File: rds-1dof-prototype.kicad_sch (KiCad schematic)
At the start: 10 parts, among them U1 Teensy4.0

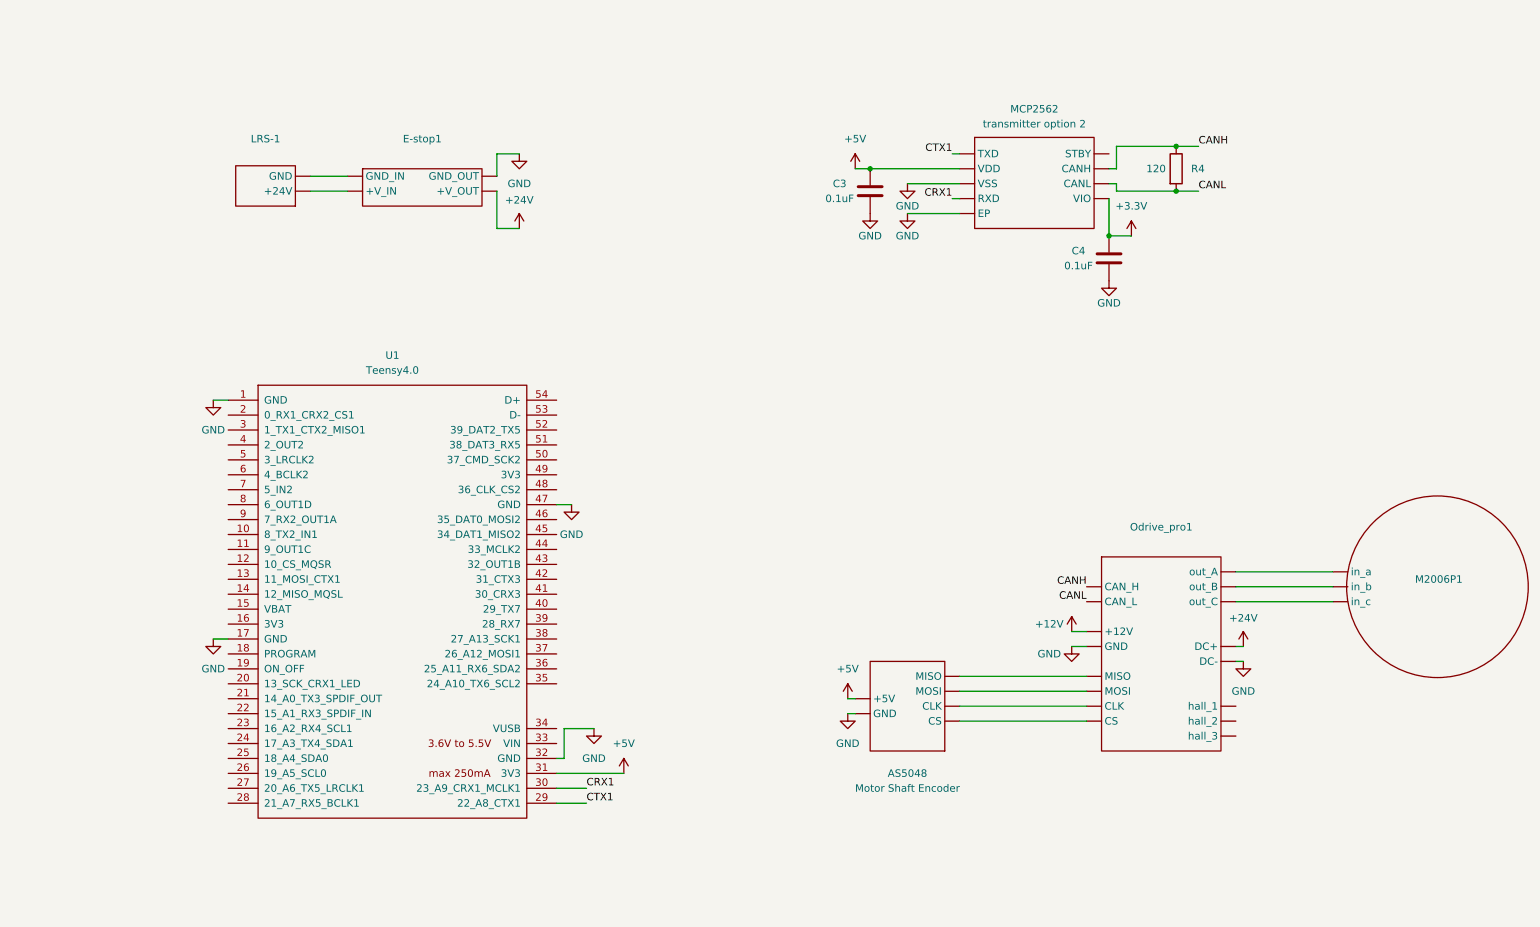
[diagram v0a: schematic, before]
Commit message: Formatting updates
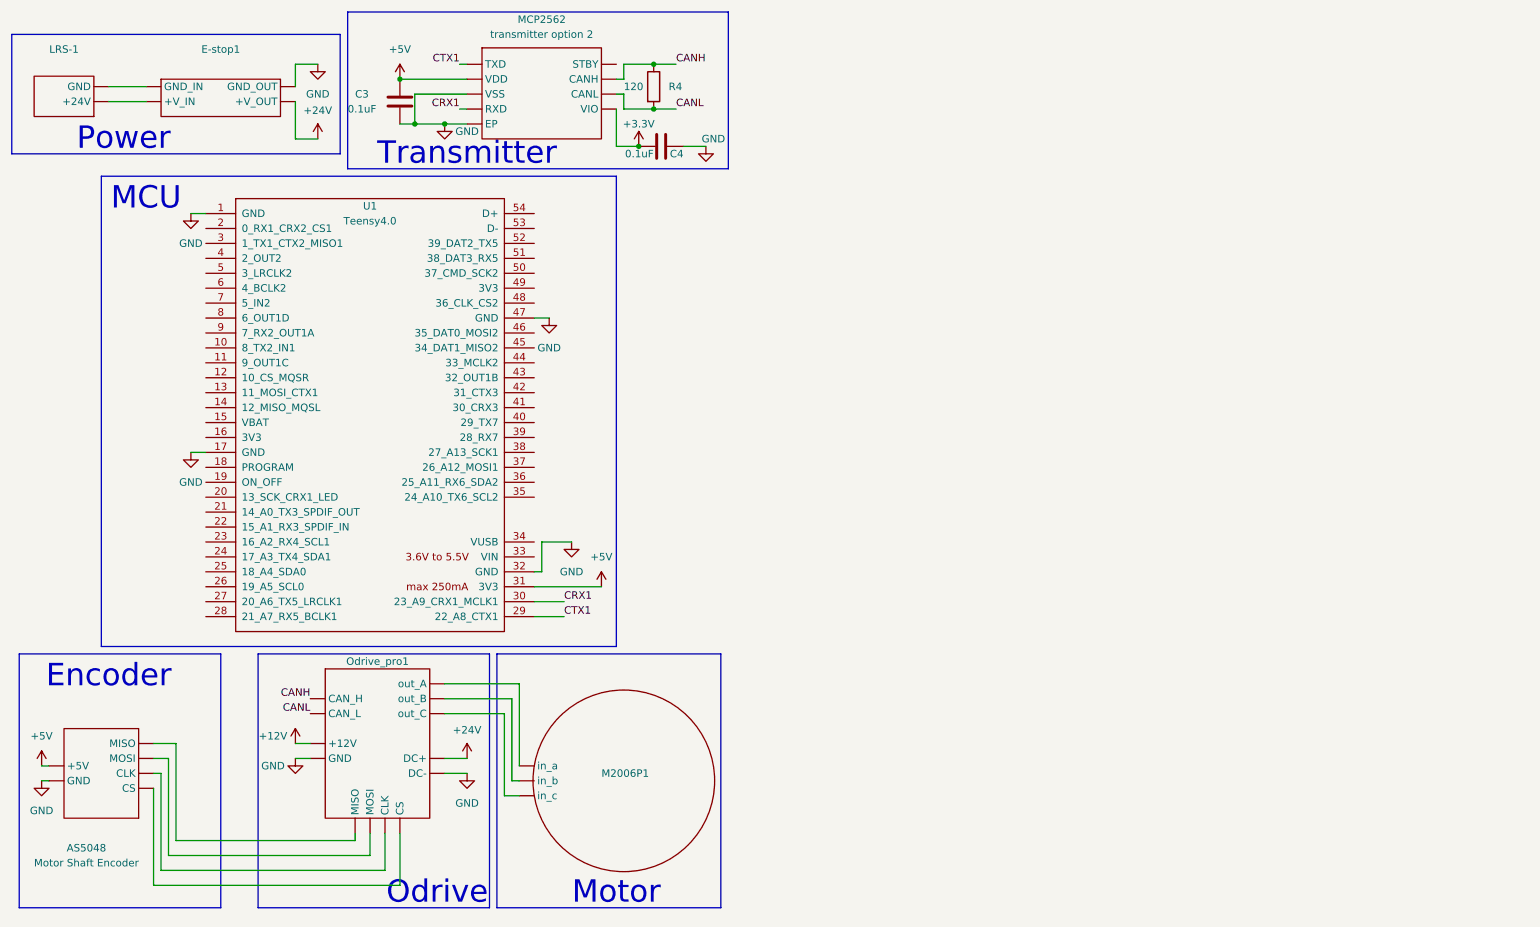
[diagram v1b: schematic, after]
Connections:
- new net: M2006P1. (in_c), Odrive_pro1. (DC-) (x2)
- new net: AS5048. (+5V), Odrive_pro1. (DC-) (x4)
- new net: E-stop1. (+V_OUT), LRS-1. (GND)
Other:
- note added: "Encoder"
- note added: "MCU"
- note added: "Motor"
- note added: "Odrive"
- note added: "Power"
- note added: "Transmitter"
- company: (none) -> RDS Speedster Team 2026
- title: (none) -> RDS 1-DOF Prototype
- moved on the sheet: AS5048, C3, C4, E-stop1, LRS-1, M2006P1, MCP2562, R4, U1
